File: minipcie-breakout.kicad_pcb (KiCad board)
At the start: 2 copper layers, 33.3 x 65 mm, 5 parts, among them J2 Conn_01x26, J3 Conn_02x26_Odd_Even, J4 Conn_01x26

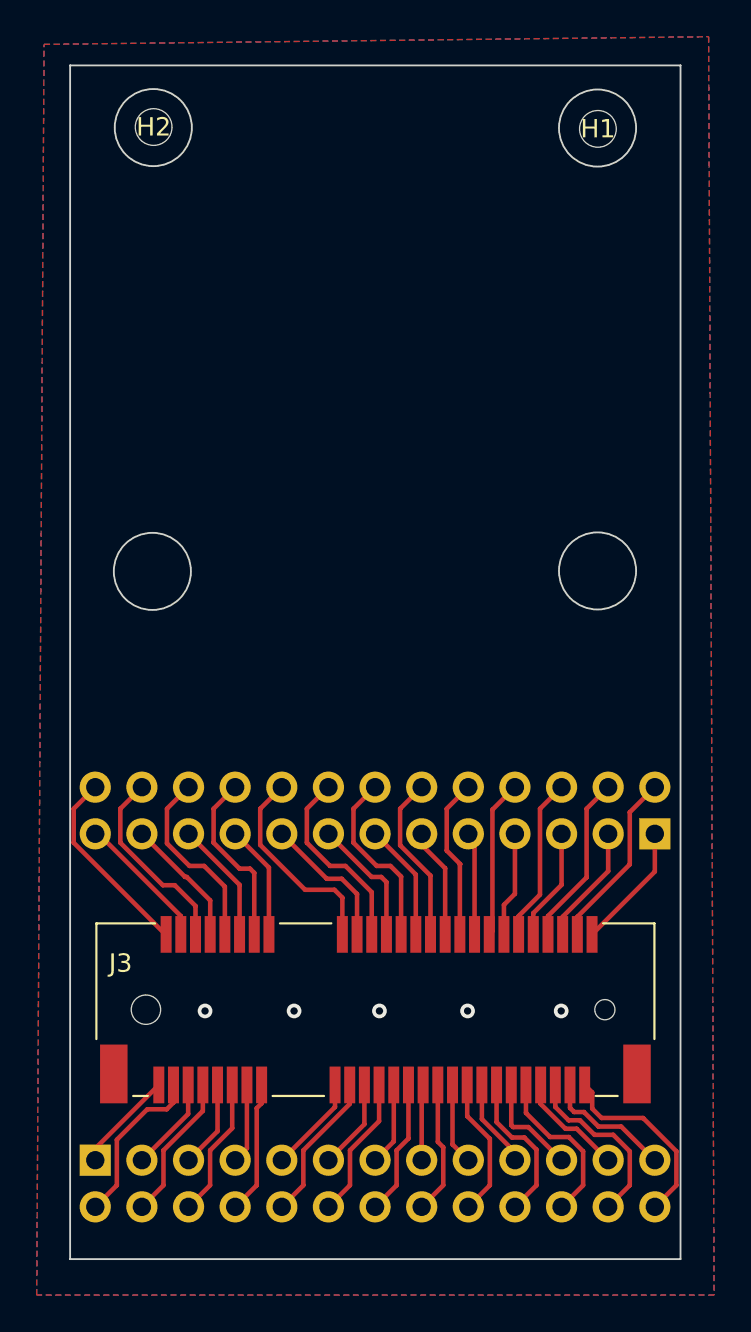
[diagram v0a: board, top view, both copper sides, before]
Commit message: latest version
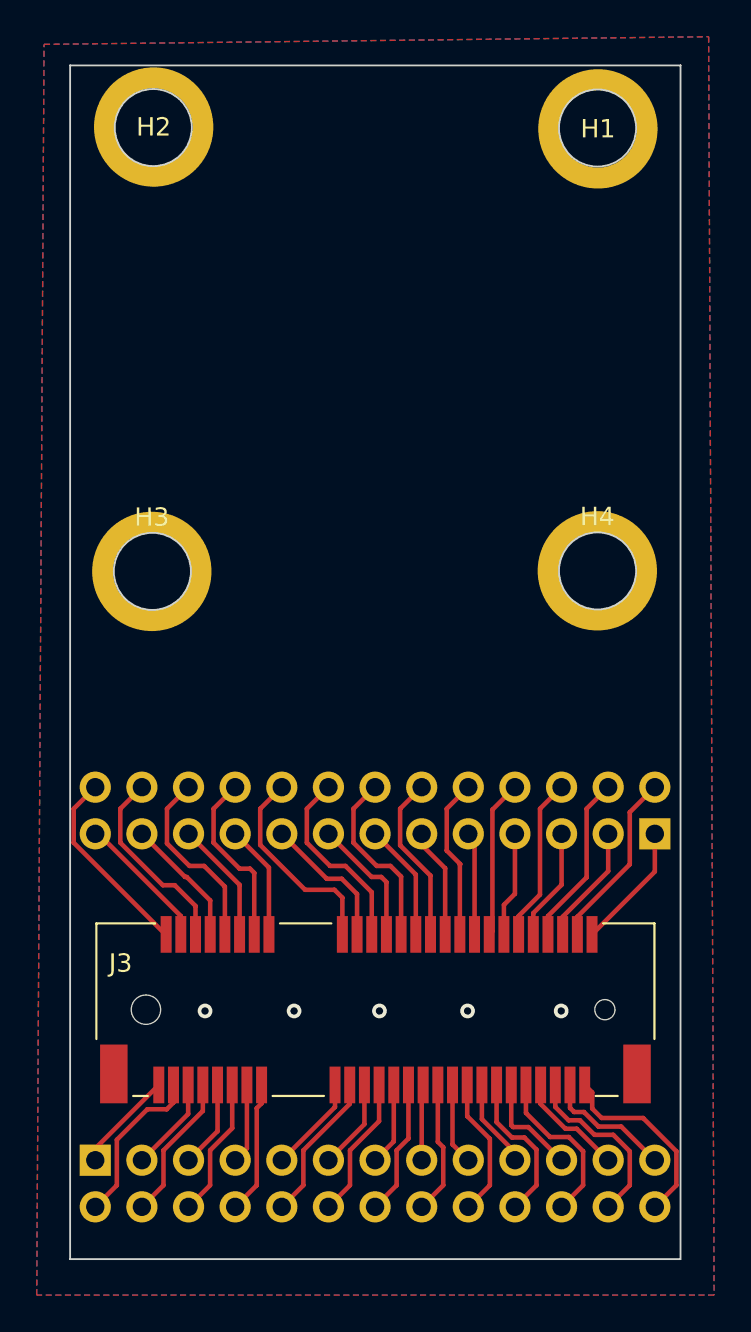
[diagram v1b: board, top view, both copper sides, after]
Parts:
- added H3: MountingHole, MountingHole:MountingHole_2mm, F.Cu at (125.0, 100.0)
- added H4: MountingHole, MountingHole:MountingHole_2mm, F.Cu at (149.3, 100.0)
